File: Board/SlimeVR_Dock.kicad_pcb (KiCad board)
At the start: 2 copper layers, 100 x 78 mm, 146 parts, among them J1Fan1 Conn_01x04_Pin, J1Temp1 Conn_01x05_Pin, J1_Control1 Conn_01x03_Pin, J1_MainPW1 USB_C_Receptacle_USB2.0_16P, J1_Monitor1 Conn_01x03_Pin, J1_Prog1 Conn_01x03_Pin, J2 USB_C_Receptacle_USB2.0_16P, J3 USB_C_Receptacle_USB2.0_16P, J4 USB_C_Receptacle_USB2.0_16P, J5 USB_C_Receptacle_USB2.0_16P, J6 USB_C_Receptacle_USB2.0_16P, J7 USB_C_Receptacle_USB2.0_16P, J8 USB_C_Receptacle_USB2.0_16P, J9 USB_C_Receptacle_USB2.0_16P, Q1 NDT452AP, Q2 BC857, Q3 BC857, Q4 BC857, Q5 BC857, Q6 BC817, U1 ESP32-C3-WROOM-02, U10 INA226, U11 AP22652W6-7, U12 INA226, U13 INA226, U14 AP22652W6-7, U15 INA226, U16 INA226, U17 74HC165, U18 74HC165, U19 74HC595, U2 CH224K, U3 XC6220B331MR, U4 TPS548A20RVER, U5 AP22652W6-7, U6 INA226, U7 INA226, U8 AP22652W6-7, U9 INA226

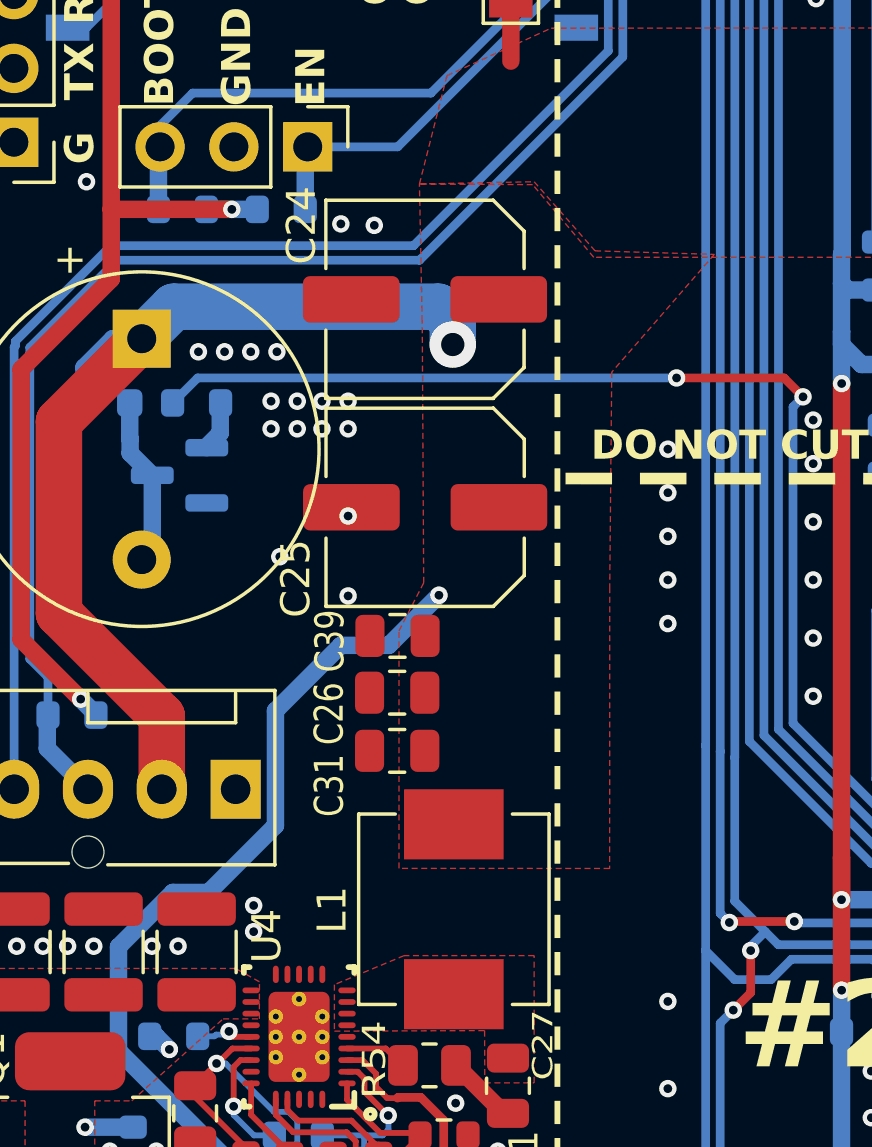
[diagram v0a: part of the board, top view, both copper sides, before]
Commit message: caps reorangement
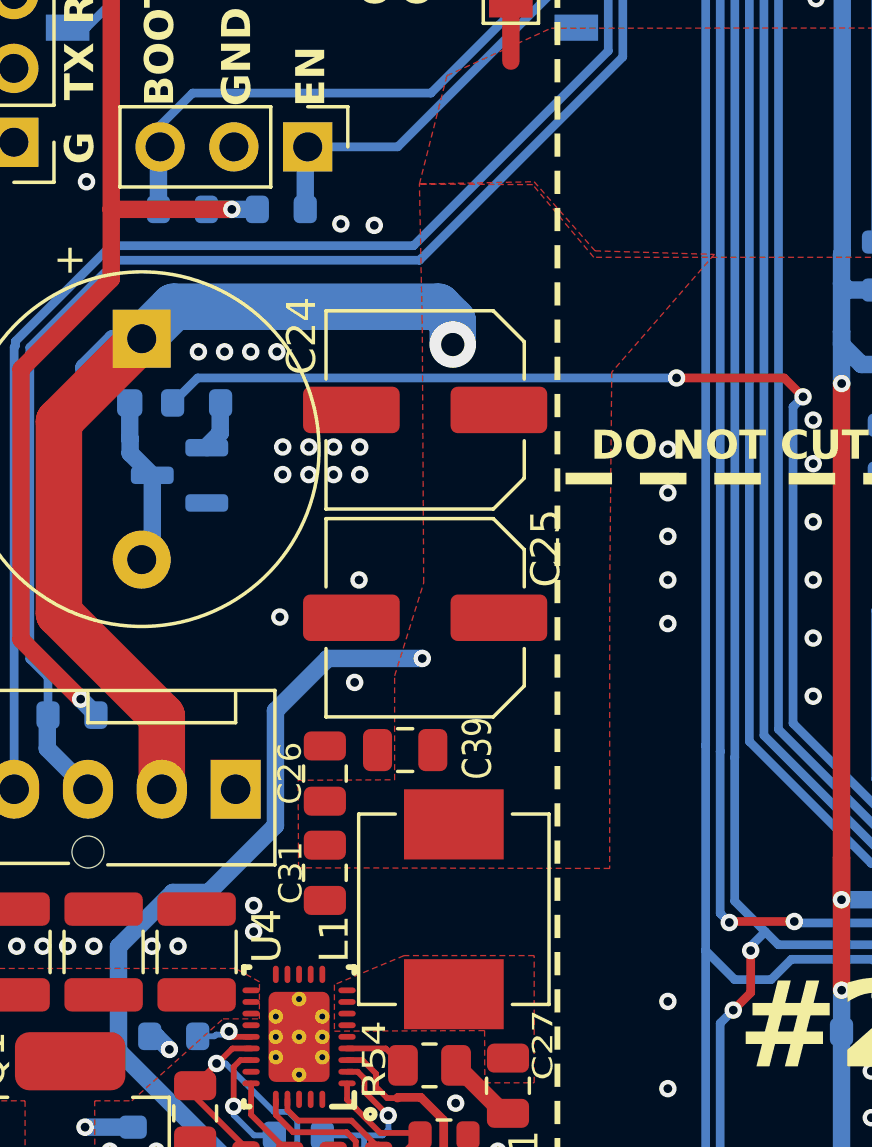
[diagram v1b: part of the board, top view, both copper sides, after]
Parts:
- moved C31 4.88 mm to (108.7, 112.1), turned to -90 degrees
- moved C39 3.94 mm to (111.5, 107.9)
- moved C24 3.80 mm to (112.2, 96.2)
- moved C25 3.80 mm to (112.2, 103.3)
- moved C26 3.73 mm to (108.7, 108.7), turned to 90 degrees
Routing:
- net 5VStepDown: track 129.9 -> 128.4 mm
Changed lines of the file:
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@@
 	(footprint "Capacitor_SMD:C_Elec_6.3x5.4"
 		(layer "F.Cu")
-		(at 112.144048 92.345536 180)
+		(at 112.15 96.15 180)
 		(descr "SMD capacitor, aluminum electrolytic nonpolar, 6.3x5.4mm")
 		(tags "capacitor electrolytic nonpolar")
@@
 	(footprint "Capacitor_SMD:C_0805_2012Metric"
 		(layer "F.Cu")
-		(at 111.1875 105.879 180)
+		(at 108.7 108.660717 90)
 		(descr "Capacitor SMD 0805 (2012 Metric), square (rectangular) end terminal, IPC-7351 nominal, (Body size source: IPC-SM-782 page 76, https://www.pcb-3d.com/wordpress/wp-content/uploads/ipc-sm-782a_amendment_1_and_2.pdf, https://docs.google.com/spreadsheets/d/1BsfQQcO9C6DZCsRaXUlFlo91Tg2WpOkGARC1WS5S8t0/edit?usp=sharing), generated with kicad-footprint-generator")
 		(tags "capacitor")
 		(property "Reference" "C26"
-			(at 2.3375 -0.721 90)
+			(at 0.010717 -1.2 90)
 			(layer "F.SilkS")
 			(effects
 				(font
-					(size 1 0.8)
+					(size 0.8 0.8)
 					(thickness 0.15)
 				)
@@
 		)
 		(property "Value" "47uF"
-			(at 0 1.68 0)
+			(at 0 1.68 90)
 			(layer "F.Fab")
 			(effects
@@
 		)
 		(property "Datasheet" ""
-			(at 0 0 0)
+			(at 0 0 90)
 			(layer "F.Fab")
 			(hide yes)
@@
 		)
 		(property "Description" "Unpolarized capacitor"
-			(at 0 0 0)
+			(at 0 0 90)
 			(layer "F.Fab")
 			(hide yes)
@@
 		(duplicate_pad_numbers_are_jumpers no)
 		(fp_line
-			(start -0.261252 0.735)
-			(end 0.261252 0.735)
+			(start -0.261252 -0.735)
+			(end 0.261252 -0.735)
 			(stroke
 				(width 0.12)
@@
 		)
 		(fp_line
-			(start -0.261252 -0.735)
-			(end 0.261252 -0.735)
+			(start -0.261252 0.735)
+			(end 0.261252 0.735)
 			(stroke
 				(width 0.12)
@@
 		)
 		(fp_text user "${REFERENCE}"
-			(at 0 0 0)
+			(at 0 0 90)
 			(layer "F.Fab")
 			(effects
@@
 		)
 		(pad "1" smd roundrect
-			(at -0.95 0 180)
+			(at -0.95 0 90)
 			(size 1 1.45)
 			(layers "F.Cu" "F.Mask" "F.Paste")
@@
 		)
 		(pad "2" smd roundrect
-			(at 0.95 0 180)
+			(at 0.95 0 90)
 			(size 1 1.45)
 			(layers "F.Cu" "F.Mask" "F.Paste")
@@
 	(footprint "Capacitor_SMD:C_0805_2012Metric"
 		(layer "F.Cu")
-		(at 111.1875 107.879 180)
+		(at 108.7 112.075 -90)
 		(descr "Capacitor SMD 0805 (2012 Metric), square (rectangular) end terminal, IPC-7351 nominal, (Body size source: IPC-SM-782 page 76, https://www.pcb-3d.com/wordpress/wp-content/uploads/ipc-sm-782a_amendment_1_and_2.pdf, https://docs.google.com/spreadsheets/d/1BsfQQcO9C6DZCsRaXUlFlo91Tg2WpOkGARC1WS5S8t0/edit?usp=sharing), generated with kicad-footprint-generator")
 		(tags "capacitor")
 		(property "Reference" "C31"
-			(at 2.331842 -1.192804 90)
+			(at 0 1.175 90)
 			(layer "F.SilkS")
 			(effects
 				(font
-					(size 1 0.8)
+					(size 0.8 0.8)
 					(thickness 0.15)
 				)
@@
 		)
 		(property "Value" "47uF"
-			(at 0 1.68 0)
+			(at 0 1.68 90)
 			(layer "F.Fab")
 			(effects
@@
 		)
 		(property "Datasheet" ""
-			(at 0 0 0)
+			(at 0 0 90)
 			(layer "F.Fab")
 			(hide yes)
@@
 		)
 		(property "Description" "Unpolarized capacitor"
-			(at 0 0 0)
+			(at 0 0 90)
 			(layer "F.Fab")
 			(hide yes)
@@
 		)
 		(fp_text user "${REFERENCE}"
-			(at 0 0 0)
+			(at 0 0 90)
 			(layer "F.Fab")
 			(effects
@@
 		)
 		(pad "1" smd roundrect
-			(at -0.95 0 180)
+			(at -0.95 0 270)
 			(size 1 1.45)
 			(layers "F.Cu" "F.Mask" "F.Paste")
@@
 		)
 		(pad "2" smd roundrect
-			(at 0.95 0 180)
+			(at 0.95 0 270)
 			(size 1 1.45)
 			(layers "F.Cu" "F.Mask" "F.Paste")
@@
 	(footprint "Capacitor_SMD:C_Elec_6.3x5.4"
 		(layer "F.Cu")
-		(at 112.15 99.5 180)
+		(at 112.15 103.3 180)
 		(descr "SMD capacitor, aluminum electrolytic nonpolar, 6.3x5.4mm")
 		(tags "capacitor electrolytic nonpolar")
 		(property "Reference" "C25"
-			(at 4.45 -2.452 90)
+			(at -4.150503 2.390925 90)
 			(layer "F.SilkS")
 			(effects
@@
 		(tags "inductor vishay ihlp smd")
 		(property "Reference" "L1"
-			(at -0.021 -4.1875 90)
+			(at -1.021 -4.1125 90)
 			(layer "F.SilkS")
 			(effects
@@
 	(footprint "Capacitor_SMD:C_0805_2012Metric"
 		(layer "F.Cu")
-		(at 111.2 103.925)
+		(at 111.462601 107.852176)
 		(descr "Capacitor SMD 0805 (2012 Metric), square (rectangular) end terminal, IPC-7351 nominal, (Body size source: IPC-SM-782 page 76, https://www.pcb-3d.com/wordpress/wp-content/uploads/ipc-sm-782a_amendment_1_and_2.pdf, https://docs.google.com/spreadsheets/d/1BsfQQcO9C6DZCsRaXUlFlo91Tg2WpOkGARC1WS5S8t0/edit?usp=sharing)")
 		(tags "capacitor")
 		(property "Reference" "C39"
-			(at -2.325 0.175 90)
+			(at 2.486848 -0.063741 90)
 			(layer "F.SilkS")
 			(effects
@@
 	)
 	(via
-		(at 108.6 95.85)
+		(at 109 97.425)
 		(size 0.6)
 		(drill 0.3)
@@
 	)
 	(via
-		(at 109.5 95.85)
+		(at 109.9 97.425)
 		(size 0.6)
 		(drill 0.3)
@@
 	)
 	(via
-		(at 107.75 95.85)
+		(at 108.15 97.425)
 		(size 0.6)
 		(drill 0.3)
@@
 	)
 	(via
-		(at 107.15 101.2)
+		(at 107.15 103.275)
 		(size 0.6)
 		(drill 0.3)
@@
 	)
 	(via
-		(at 107.75 96.8)
+		(at 108.15 98.375)
 		(size 0.6)
 		(drill 0.3)
@@
 	)
 	(via
-		(at 109.5 102.55)
+		(at 109.725 105.525)
 		(size 0.6)
 		(drill 0.3)
@@
 	)
 	(via
-		(at 108.6 96.8)
+		(at 109 98.375)
 		(size 0.6)
 		(drill 0.3)
@@
 	)
 	(via
-		(at 109.5 99.8)
+		(at 109.875 102)
 		(size 0.6)
 		(drill 0.3)
@@
 	)
 	(via
-		(at 106.85 95.85)
+		(at 107.25 97.425)
 		(size 0.6)
 		(drill 0.3)
@@
 	)
 	(via
-		(at 109.5 96.8)
+		(at 109.9 98.375)
 		(size 0.6)
 		(drill 0.3)
@@
 	)
 	(via
-		(at 106.85 96.8)
+		(at 107.25 98.375)
 		(size 0.6)
 		(drill 0.3)
@@
 	)
 	(via
-		(at 112.625 102.525)
+		(at 112.05 104.7)
 		(size 0.6)
 		(drill 0.3)
@@
 	)
 	(segment
-		(start 104.7 112.75)
-		(end 103.468629 112.75)
-		(width 0.6)
-		(layer "B.Cu")
-		(net "5VStepDown")
-	)
-	(segment
 		(start 146.7196 90.5804)
 		(end 146.7196 92.72365)
@@
 	)
 	(segment
-		(start 101.6 114.618629)
-		(end 101.6 118.2)
-		(width 0.6)
-		(layer "B.Cu")
-		(net "5VStepDown")
-	)
-	(segment
 		(start 189.125 90.025)
 		(end 188.5 89.4)
@@
 	)
 	(segment
-		(start 112.625 102.525)
-		(end 110.9 104.25)
-		(width 0.6)
-		(layer "B.Cu")
-		(net "5VStepDown")
-	)
-	(segment
-		(start 101.6 118.2)
-		(end 105.95 122.55)
+		(start 107 106.5)
+		(end 107 110.45)
 		(width 0.6)
 		(layer "B.Cu")
@@
 	)
 	(segment
-		(start 107 110.45)
-		(end 104.7 112.75)
-		(width 0.6)
-		(layer "B.Cu")
-		(net "5VStepDown")
-	)
-	(segment
 		(start 147.049999 91.275001)
 		(end 147.225 91.1)
@@
 	)
 	(segment
-		(start 103.468629 112.75)
-		(end 101.6 114.618629)
-		(width 0.6)
-		(layer "B.Cu")
-		(net "5VStepDown")
-	)
-	(segment
 		(start 167.049999 90.169607)
 		(end 167.049272 90.16888)
@@
 	)
 	(segment
+		(start 103.468629 112.75)
+		(end 101.6 114.618629)
+		(width 0.6)
+		(layer "B.Cu")
+		(net "5VStepDown")
+	)
+	(segment
 		(start 147.049999 91.7)
 		(end 147.049999 90.250001)
@@
 	)
 	(segment
-		(start 105.95 122.55)
-		(end 108.0875 122.55)
+		(start 112.05 104.7)
+		(end 108.8 104.7)
 		(width 0.6)
 		(layer "B.Cu")
@@
 	)
 	(segment
-		(start 109.25 104.25)
+		(start 101.6 114.618629)
+		(end 101.6 118.2)
+		(width 0.6)
+		(layer "B.Cu")
+		(net "5VStepDown")
+	)
+	(segment
+		(start 108.8 104.7)
 		(end 107 106.5)
 		(width 0.6)
@@
 	)
 	(segment
-		(start 107 106.5)
-		(end 107 110.45)
+		(start 104.7 112.75)
+		(end 103.468629 112.75)
 		(width 0.6)
 		(layer "B.Cu")
@@
 	)
 	(segment
+		(start 105.95 122.55)
+		(end 108.0875 122.55)
+		(width 0.6)
+		(layer "B.Cu")
+		(net "5VStepDown")
+	)
+	(segment
 		(start 131.749998 91.9)
 		(end 131.749998 90.150002)
@@
 	)
 	(segment
-		(start 110.9 104.25)
-		(end 109.25 104.25)
+		(start 107 110.45)
+		(end 104.7 112.75)
 		(width 0.6)
 		(layer "B.Cu")
@@
 	)
 	(segment
+		(start 101.6 118.2)
+		(end 105.95 122.55)
+		(width 0.6)
+		(layer "B.Cu")
+		(net "5VStepDown")
+	)
+	(segment
 		(start 128.9 129.7)
 		(end 127.6 129.7)
@@
 		(polygon
 			(pts
-				(xy 118.569831 94.850187) (xy 118.5 102.248) (xy 118.497353 111.924983) (xy 111.25 111.923) (xy 111.25 103.75)
-				(xy 112.1 102.099849) (xy 112.05 93.1) (xy 112.046113 93.097309) (xy 111.953392 88.377532) (xy 115.9 88.3)
-				(xy 117.996112 90.67782) (xy 122.1 90.8)
+				(xy 118.569831 94.850187) (xy 118.5 102.248) (xy 118.497353 111.924983) (xy 107.794322 111.903874)
+				(xy 107.779573 108.891256) (xy 111.1 108.875) (xy 111.1 105.3) (xy 112.1 102.099849) (xy 112.05 93.1)
+				(xy 112.046113 93.097309) (xy 111.953392 88.377532) (xy 115.9 88.3) (xy 117.996112 90.67782) (xy 122.1 90.8)
 			)
 		)
